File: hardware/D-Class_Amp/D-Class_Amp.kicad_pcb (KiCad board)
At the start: 2 copper layers, 180 x 65 mm, 99 parts, among them J101 P_IN, J102 AudioJack2, Q501 PHP23NQ11T, Q502 PHP23NQ11T, Q503 PHP23NQ11T, Q504 PHP23NQ11T, U101 NCP1117-12_TO252, U102 MCP1799T-5002H_TT, U201 LM324, U301 TL972, U302 LMV393, U501 IR21834, U502 IR21834

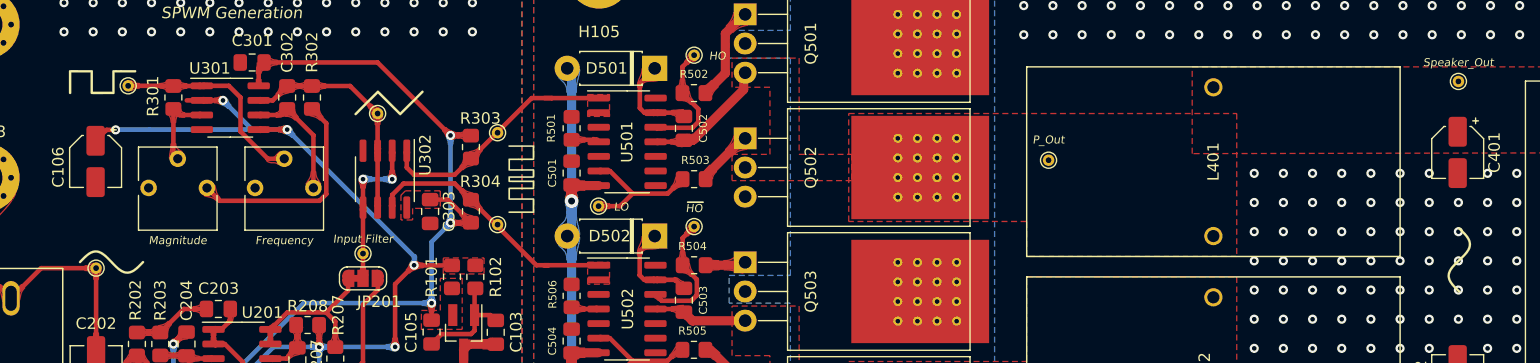
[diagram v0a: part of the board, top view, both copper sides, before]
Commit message: hopefully fixed the repo
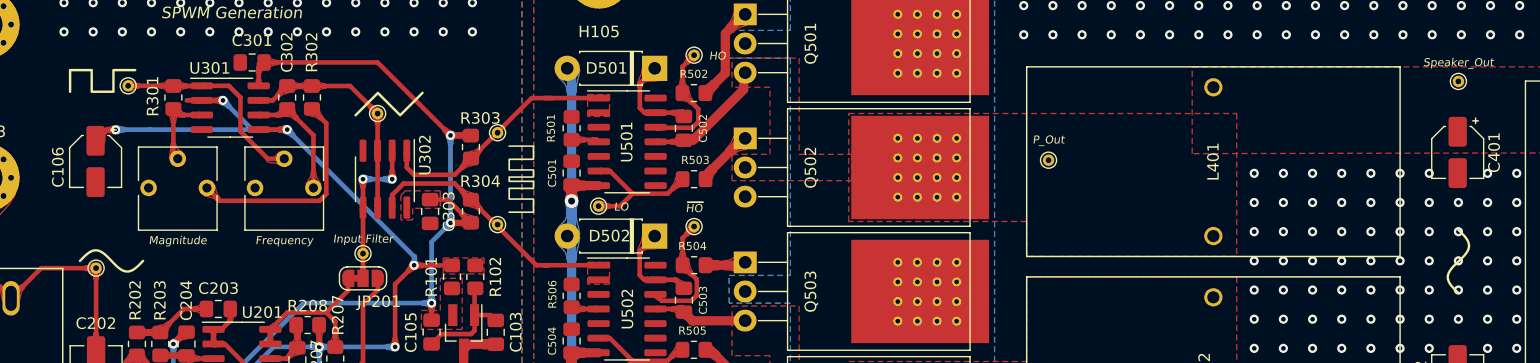
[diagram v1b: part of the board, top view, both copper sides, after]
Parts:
- removed the G*** at (216.7, 97.1)
- removed the G*** at (99.4, 97.3)
- added G***: LOGO, silk_art:sine, F.Cu at (99.4, 97.2)
- added G***: LOGO, silk_art:sine, F.Cu at (216.7, 97.2)
- C106: value 100u -> 100u 6.3V
- moved G*** 0.76 mm to (240.7, 98.5)
- moved G*** 0.10 mm to (98.5, 81.6)
- moved G*** 0.10 mm to (123.5, 83.6)
